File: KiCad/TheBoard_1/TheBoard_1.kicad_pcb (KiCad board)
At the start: 2 copper layers, 31 parts, among them J1 Conn_01x16_Female, J2 Conn_01x16_Female, J3 Conn_01x01_Male, J4 Conn_01x01_Male, J5 Conn_01x01_Male, J6 Conn_01x01_Male, U1 TL431D, U2 TL431D, U3 YAAJ_WeAct_BlackPill_Part_Lik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, U4 TL431D, U5 TL431D

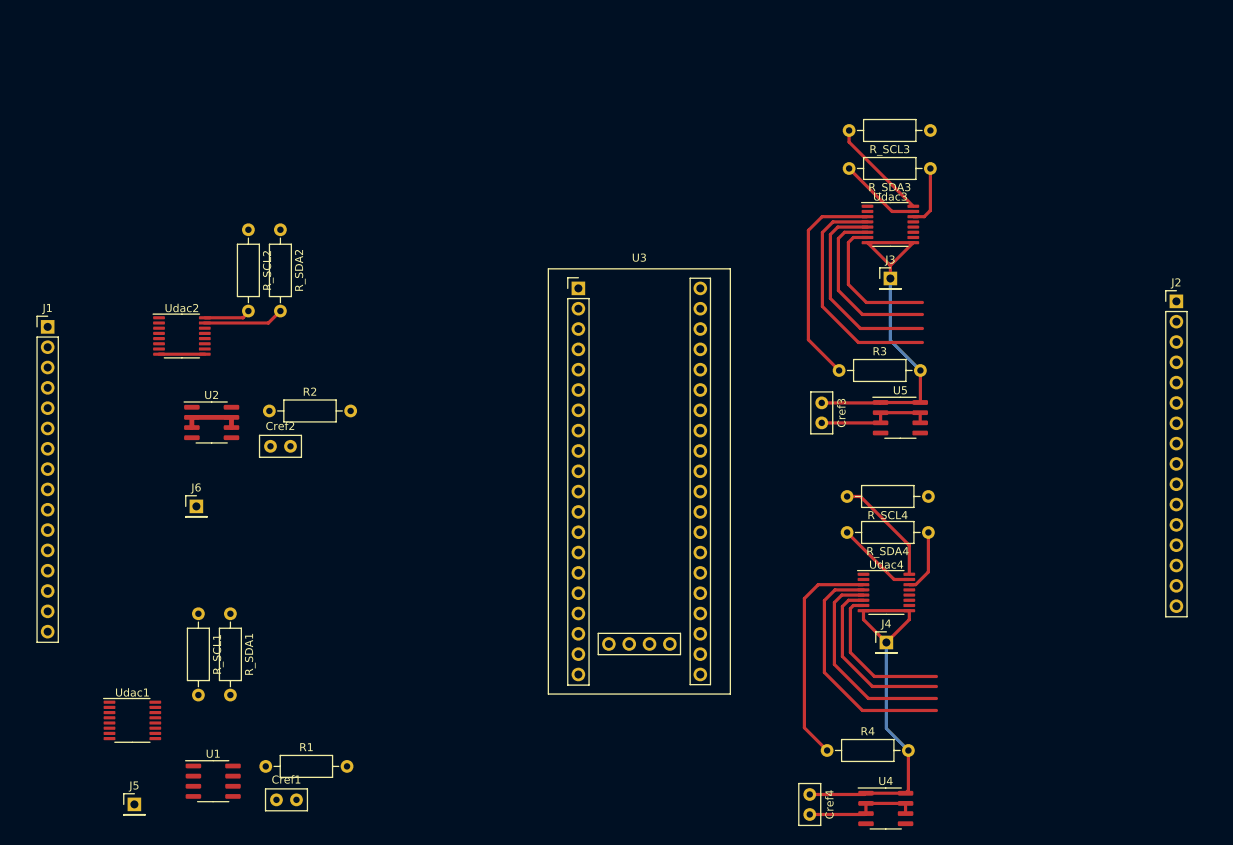
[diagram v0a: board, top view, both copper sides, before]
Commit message: progress
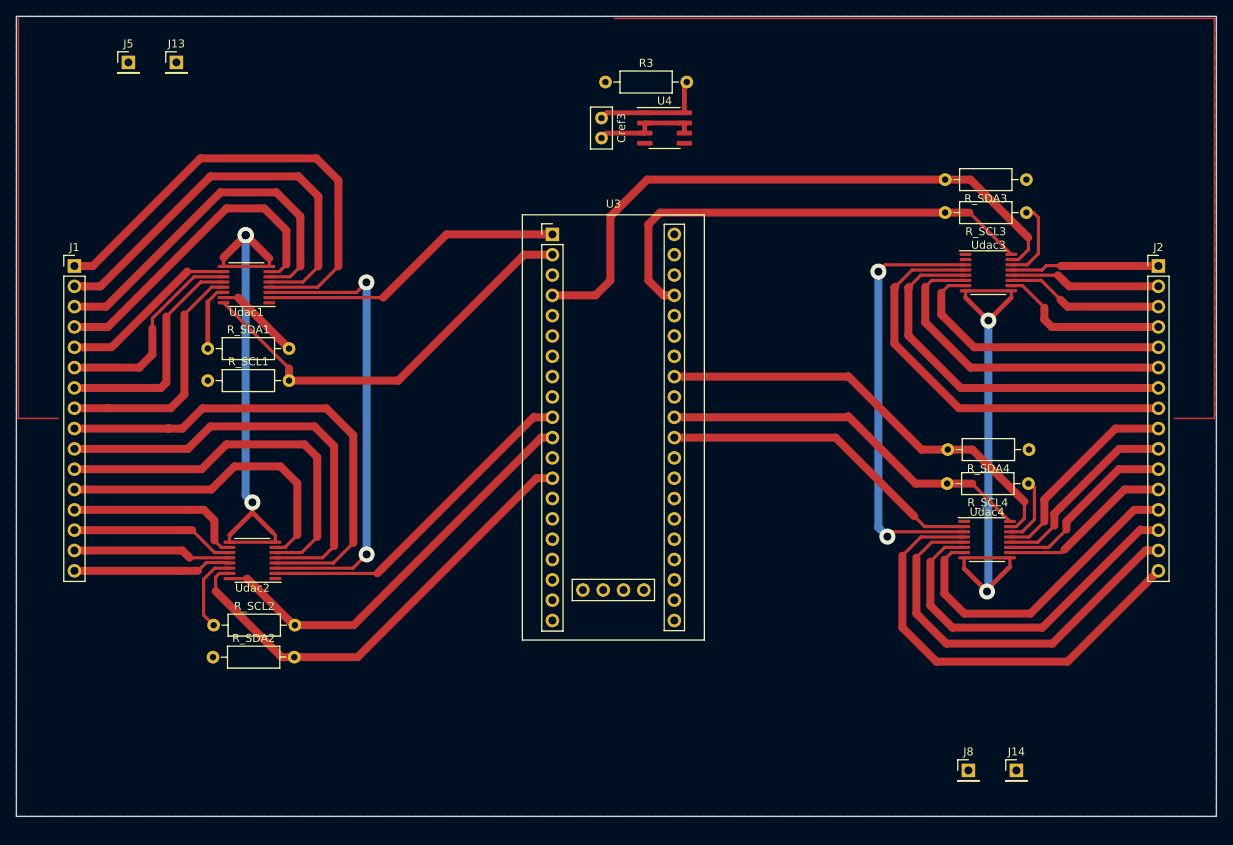
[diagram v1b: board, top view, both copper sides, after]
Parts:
- removed Cref1, Cref2, Cref4: 100n, Capacitor_THT:C_Disc_D5.0mm_W2.5mm_P2.50mm
- removed J3, J4, J6: Conn_01x01_Male, Connector_PinHeader_2.54mm:PinHeader_1x01_P2.54mm_Vertical
- removed R1, R2, R4: R, Resistor_THT:R_Axial_DIN0207_L6.3mm_D2.5mm_P10.16mm_Horizontal
- removed U1, U2, U5: TL431D, Package_SO:SOIC-8_3.9x4.9mm_P1.27mm
- added J13: Conn_01x01_Male, Connector_PinHeader_2.54mm:PinHeader_1x01_P2.54mm_Vertical, F.Cu at (99.5, 53.0)
- added J14: Conn_01x01_Male, Connector_PinHeader_2.54mm:PinHeader_1x01_P2.54mm_Vertical, F.Cu at (204.5, 141.5)
- added J8: Conn_01x01_Male, Connector_PinHeader_2.54mm:PinHeader_1x01_P2.54mm_Vertical, F.Cu at (198.5, 141.5)
- moved J5 92.8 mm to (93.5, 53.0)
- moved U4 89.4 mm to (160.5, 61.2)
- moved Udac1 56.3 mm to (108.2, 80.8), turned to 180 degrees
- moved R_SDA2 54.1 mm to (104.1, 127.3), turned to 0 degrees
- moved R_SCL2 49.6 mm to (104.2, 123.3), turned to 0 degrees
- moved R3 46.4 mm to (153.1, 55.5)
- moved Cref3 45.0 mm to (152.6, 60.0)
- moved R_SDA1 33.3 mm to (103.4, 88.8), turned to 0 degrees
- moved Udac2 29.4 mm to (109.0, 115.2), turned to 180 degrees
- moved R_SCL1 29.2 mm to (103.4, 92.8), turned to 0 degrees
- moved R_SDA4 16.3 mm to (206.1, 101.4)
- moved R_SCL3 15.8 mm to (205.8, 71.8)
- moved Udac4 14.2 mm to (200.8, 112.7)
- moved Udac3 13.6 mm to (201.0, 79.3)
- moved R_SCL4 12.6 mm to (206.0, 105.7)
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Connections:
- J1 pad 4: Net-(J1-Pad4) -> Net-(Udac1-Pad7)
- J1 pad 5: Net-(J1-Pad5) -> Net-(Udac1-Pad10)
- J1 pad 6: Net-(J1-Pad6) -> Net-(Udac1-Pad11)
- J1 pad 7: Net-(J1-Pad7) -> Net-(Udac1-Pad12)
- J1 pad 8: Net-(J1-Pad8) -> Net-(Udac1-Pad13)
- J2 pad 1: Net-(J2-Pad1) -> Net-(Udac3-Pad13)
- J2 pad 10: Net-(J2-Pad10) -> Net-(Udac4-Pad12)
- J2 pad 11: Net-(J2-Pad11) -> Net-(Udac4-Pad11)
- J2 pad 12: Net-(J2-Pad12) -> Net-(Udac4-Pad10)
- J2 pad 13: Net-(J2-Pad13) -> Net-(Udac4-Pad7)
- J2 pad 14: Net-(J2-Pad14) -> Net-(Udac4-Pad6)
- J2 pad 15: Net-(J2-Pad15) -> Net-(Udac4-Pad5)
- J2 pad 16: Net-(J2-Pad16) -> Net-(Udac4-Pad4)
- J2 pad 2: Net-(J2-Pad2) -> Net-(Udac3-Pad12)
- J2 pad 3: Net-(J2-Pad3) -> Net-(Udac3-Pad11)
- J2 pad 4: Net-(J2-Pad4) -> Net-(Udac3-Pad10)
- J2 pad 5: Net-(J2-Pad5) -> Net-(Udac3-Pad7)
- J2 pad 6: Net-(J2-Pad6) -> Net-(Udac3-Pad6)
- J2 pad 7: Net-(J2-Pad7) -> Net-(Udac3-Pad5)
- J2 pad 8: Net-(J2-Pad8) -> Net-(Udac3-Pad4)
- J2 pad 9: Net-(J2-Pad9) -> Net-(Udac4-Pad13)
- J5 pad 1: +2V5 -> +5V
- Udac1 pad 1: unconnected-(Udac1-Pad1) -> Net-(Udac1-Pad1)
- Udac1 pad 10: Net-(J1-Pad9) -> Net-(Udac1-Pad10)
- Udac1 pad 11: Net-(J1-Pad11) -> Net-(Udac1-Pad11)
- Udac1 pad 12: Net-(J1-Pad13) -> Net-(Udac1-Pad12)
- Udac1 pad 13: Net-(J1-Pad15) -> Net-(Udac1-Pad13)
- Udac1 pad 4: Net-(J1-Pad16) -> Net-(J1-Pad1)
- Udac1 pad 5: Net-(J1-Pad14) -> Net-(J1-Pad2)
- Udac1 pad 6: Net-(J1-Pad12) -> Net-(J1-Pad3)
- Udac1 pad 7: Net-(J1-Pad10) -> Net-(Udac1-Pad7)
- Udac2 pad 1: unconnected-(Udac2-Pad1) -> Net-(Udac1-Pad1)
- Udac2 pad 10: Net-(J1-Pad1) -> Net-(J1-Pad13)
- Udac2 pad 11: Net-(J1-Pad3) -> Net-(J1-Pad14)
- Udac2 pad 12: Net-(J1-Pad5) -> Net-(J1-Pad15)
- Udac2 pad 13: Net-(J1-Pad7) -> Net-(J1-Pad16)
- Udac2 pad 4: Net-(J1-Pad8) -> Net-(J1-Pad9)
- Udac2 pad 5: Net-(J1-Pad6) -> Net-(J1-Pad10)
- Udac2 pad 6: Net-(J1-Pad4) -> Net-(J1-Pad11)
- Udac2 pad 7: Net-(J1-Pad2) -> Net-(J1-Pad12)
- Udac3 pad 1: unconnected-(Udac3-Pad1) -> Net-(Udac1-Pad1)
- Udac3 pad 10: Net-(J2-Pad8) -> Net-(Udac3-Pad10)
- Udac3 pad 11: Net-(J2-Pad6) -> Net-(Udac3-Pad11)
- Udac3 pad 12: Net-(J2-Pad4) -> Net-(Udac3-Pad12)
- Udac3 pad 13: Net-(J2-Pad2) -> Net-(Udac3-Pad13)
- Udac3 pad 4: Net-(J2-Pad1) -> Net-(Udac3-Pad4)
- Udac3 pad 5: Net-(J2-Pad3) -> Net-(Udac3-Pad5)
- Udac3 pad 6: Net-(J2-Pad5) -> Net-(Udac3-Pad6)
- Udac3 pad 7: Net-(J2-Pad7) -> Net-(Udac3-Pad7)
- Udac4 pad 1: unconnected-(Udac4-Pad1) -> Net-(Udac1-Pad1)
- Udac4 pad 10: Net-(J2-Pad16) -> Net-(Udac4-Pad10)
- Udac4 pad 11: Net-(J2-Pad14) -> Net-(Udac4-Pad11)
- Udac4 pad 12: Net-(J2-Pad12) -> Net-(Udac4-Pad12)
- Udac4 pad 13: Net-(J2-Pad10) -> Net-(Udac4-Pad13)
- Udac4 pad 4: Net-(J2-Pad9) -> Net-(Udac4-Pad4)
- Udac4 pad 5: Net-(J2-Pad11) -> Net-(Udac4-Pad5)
- Udac4 pad 6: Net-(J2-Pad13) -> Net-(Udac4-Pad6)
- Udac4 pad 7: Net-(J2-Pad15) -> Net-(Udac4-Pad7)
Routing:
- net Net-(U3-Pad4): track 10.2 -> 77.3 mm
- net Net-(J1-Pad9): track 0.00 -> 61.6 mm
- net Net-(J1-Pad1): track 0.00 -> 60.2 mm
- net +5V: track 55.5 -> 113.5 mm, vias 0 -> 4
- net Net-(Udac4-Pad4): track 0.00 -> 56.1 mm
- net Net-(J1-Pad10): track 0.00 -> 55.3 mm
- net Net-(Udac3-Pad4): track 0.00 -> 53.1 mm
- net Net-(J1-Pad2): track 0.00 -> 52.9 mm
- net Net-(R_SCL1-Pad2): track 0.00 -> 52.6 mm
- net Net-(Udac4-Pad5): track 0.00 -> 50.4 mm
- net Net-(R_SDA2-Pad2): track 10.1 -> 58.5 mm
- net Net-(J1-Pad11): track 0.00 -> 48.3 mm
- net +2V5: track 98.8 -> 147.0 mm, vias 0 -> 5
- net Net-(Udac3-Pad5): track 0.00 -> 47.7 mm
- net Net-(R_SCL2-Pad2): track 5.90 -> 52.5 mm
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- added copper zone on B.Cu, net GND
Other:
- board outline added: 150 x 100 mm
